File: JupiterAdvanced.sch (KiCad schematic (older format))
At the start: 224 parts, among them SW1 SW_Push, U1 PRTR5V0U2X, U10 ATmega32U4-AU, Y1 16MHz

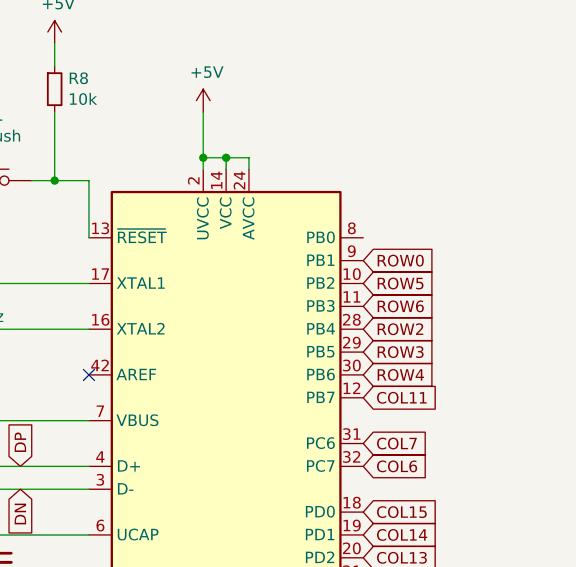
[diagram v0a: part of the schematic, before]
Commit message: Rerouting for atmega32u4 complete
and its a complete mess...
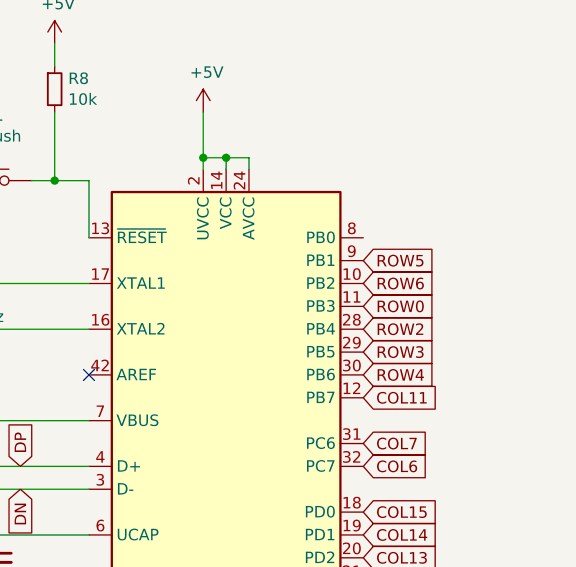
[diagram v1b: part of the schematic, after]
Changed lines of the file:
@@
 Text GLabel 12300 3550 2    50   Input ~ 0
 COL15
+Text GLabel 12300 2550 2    50   Input ~ 0
+ROW6
 Text GLabel 12300 2650 2    50   Input ~ 0
-ROW6
-Text GLabel 12300 2450 2    50   Input ~ 0
 ROW0
 Text GLabel 12300 3250 2    50   Input ~ 0
@@
 Wire Wire Line
 	9850 2450 9750 2450
-Text GLabel 12300 2550 2    50   Input ~ 0
+Text GLabel 12300 2450 2    50   Input ~ 0
 ROW5
 $EndSCHEMATC
